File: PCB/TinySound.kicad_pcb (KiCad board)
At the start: 4 copper layers, 15.2 x 15.7 mm, 23 parts, among them J1 Conn_01x02, J2 Conn_01x02, J3 Micro_SD_Card_Det, J4 Conn_01x04, J5 Conn_01x02, U1 MAX98360AENL+, U2 STM32G030KxT, U3 MAX98360xxxB+

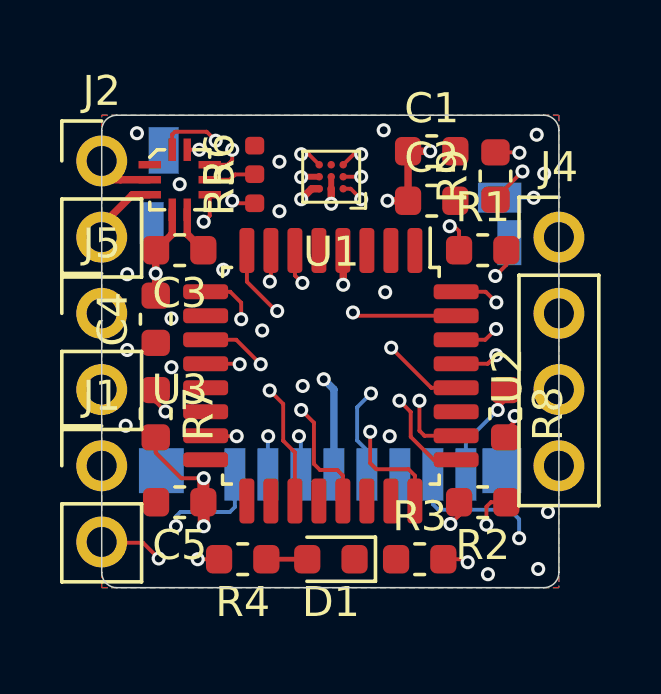
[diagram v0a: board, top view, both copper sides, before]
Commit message: [PCB] Minor tweaks
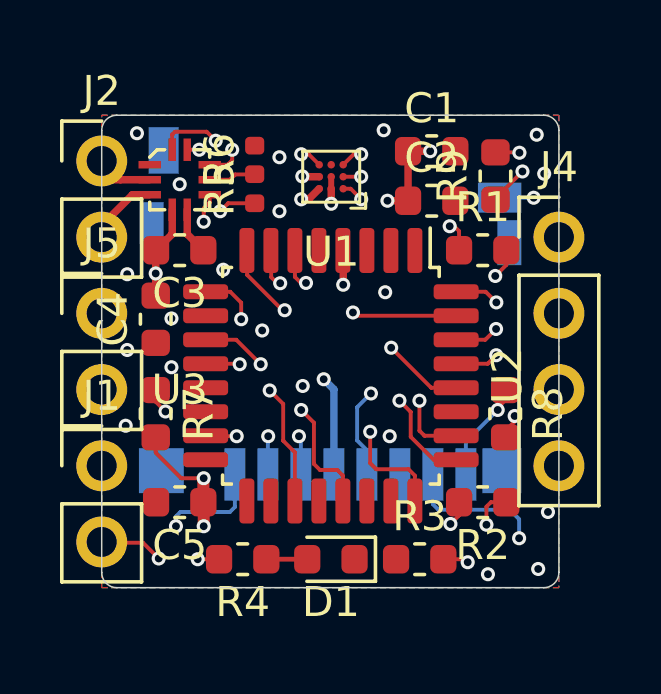
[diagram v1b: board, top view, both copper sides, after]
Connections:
- J4 pad 2: /NRST -> /SWDIO
- J4 pad 3: /SWDIO -> /SWCLK_BOOT0_WAKEUP
- J4 pad 4: /SWCLK_BOOT0_WAKEUP -> /NRST
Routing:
- net /NRST: track 28.6 -> 17.2 mm
- net /SWDIO: track 9.93 -> 11.6 mm
- net /SWCLK_BOOT0_WAKEUP: track 22.7 -> 24.1 mm
- net /AU_BCLK: track 17.7 -> 16.3 mm
- net +3V3: track 73.5 -> 74.1 mm
